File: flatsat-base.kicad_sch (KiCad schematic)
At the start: 11 parts, among them J1 xf2m-2415-1a-symbols, J10 Conn_01x24_Male, J11 Conn_02x05_Odd_Even, J12 Conn_02x05_Odd_Even, J13 Conn_01x10_Male, J3 XF2M-1015-1A-symbols, J4 XF2M-1015-1A-symbols, J5 XF2M-1015-1A-symbols, J6 XF2M-1015-1A-symbols, J7 XF2M-1015-1A-symbols, J8 XF2M-1015-1A-symbols

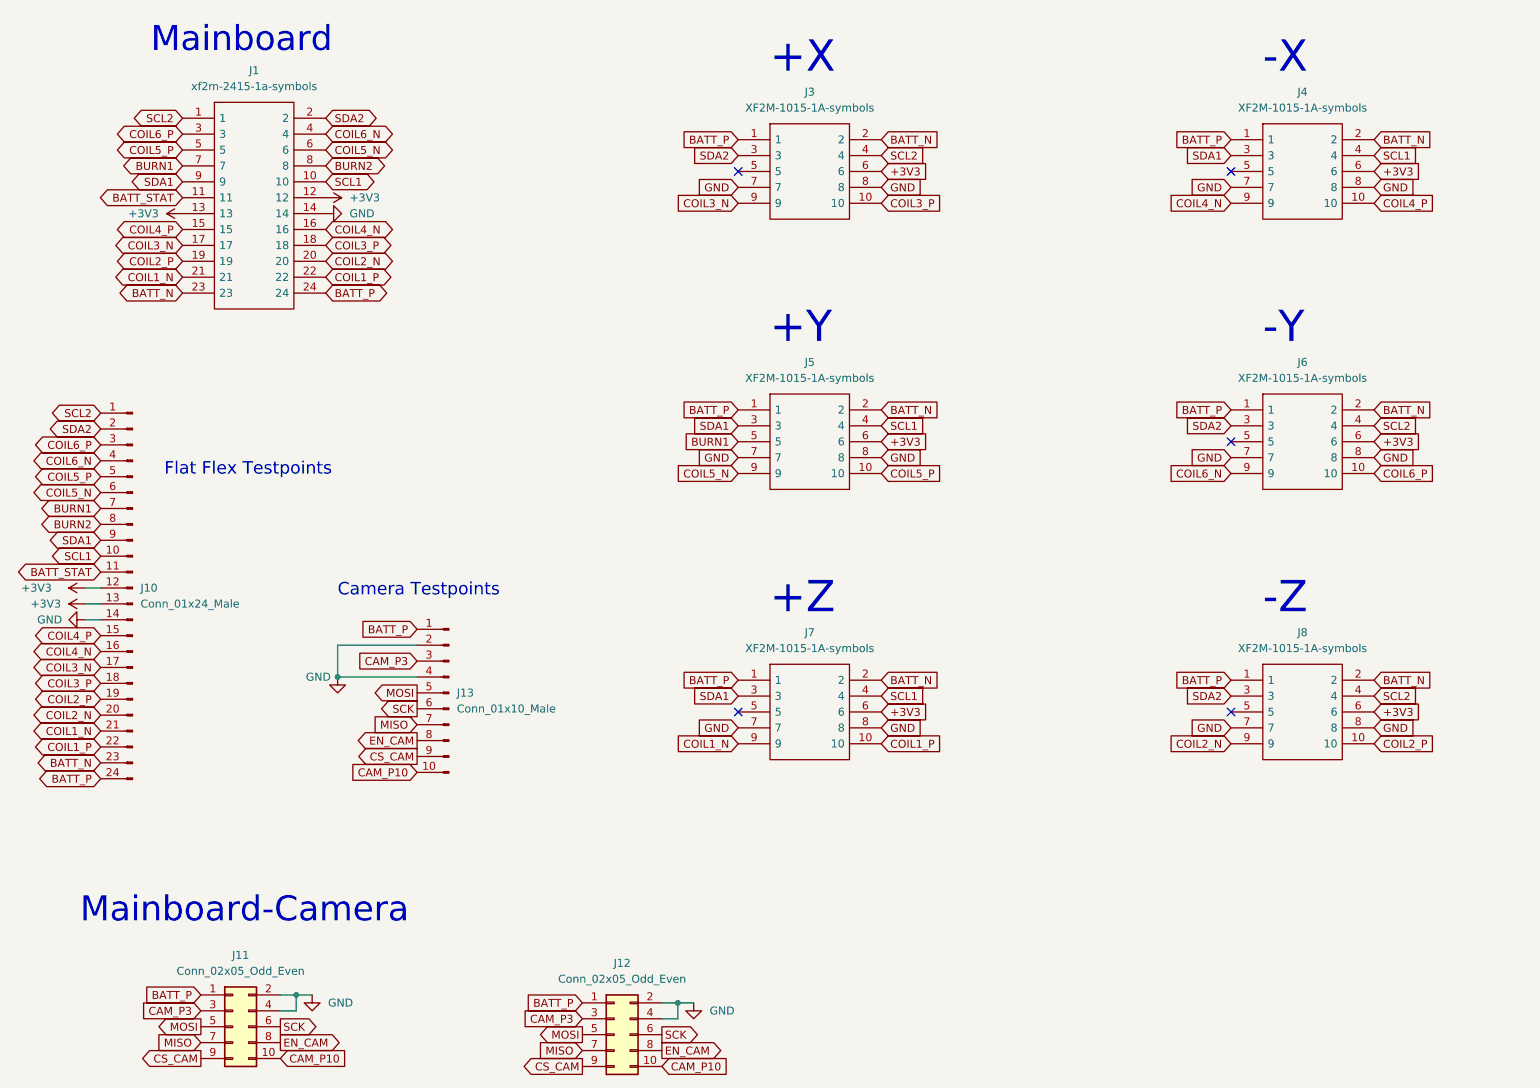
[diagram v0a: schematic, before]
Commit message: Partially routed
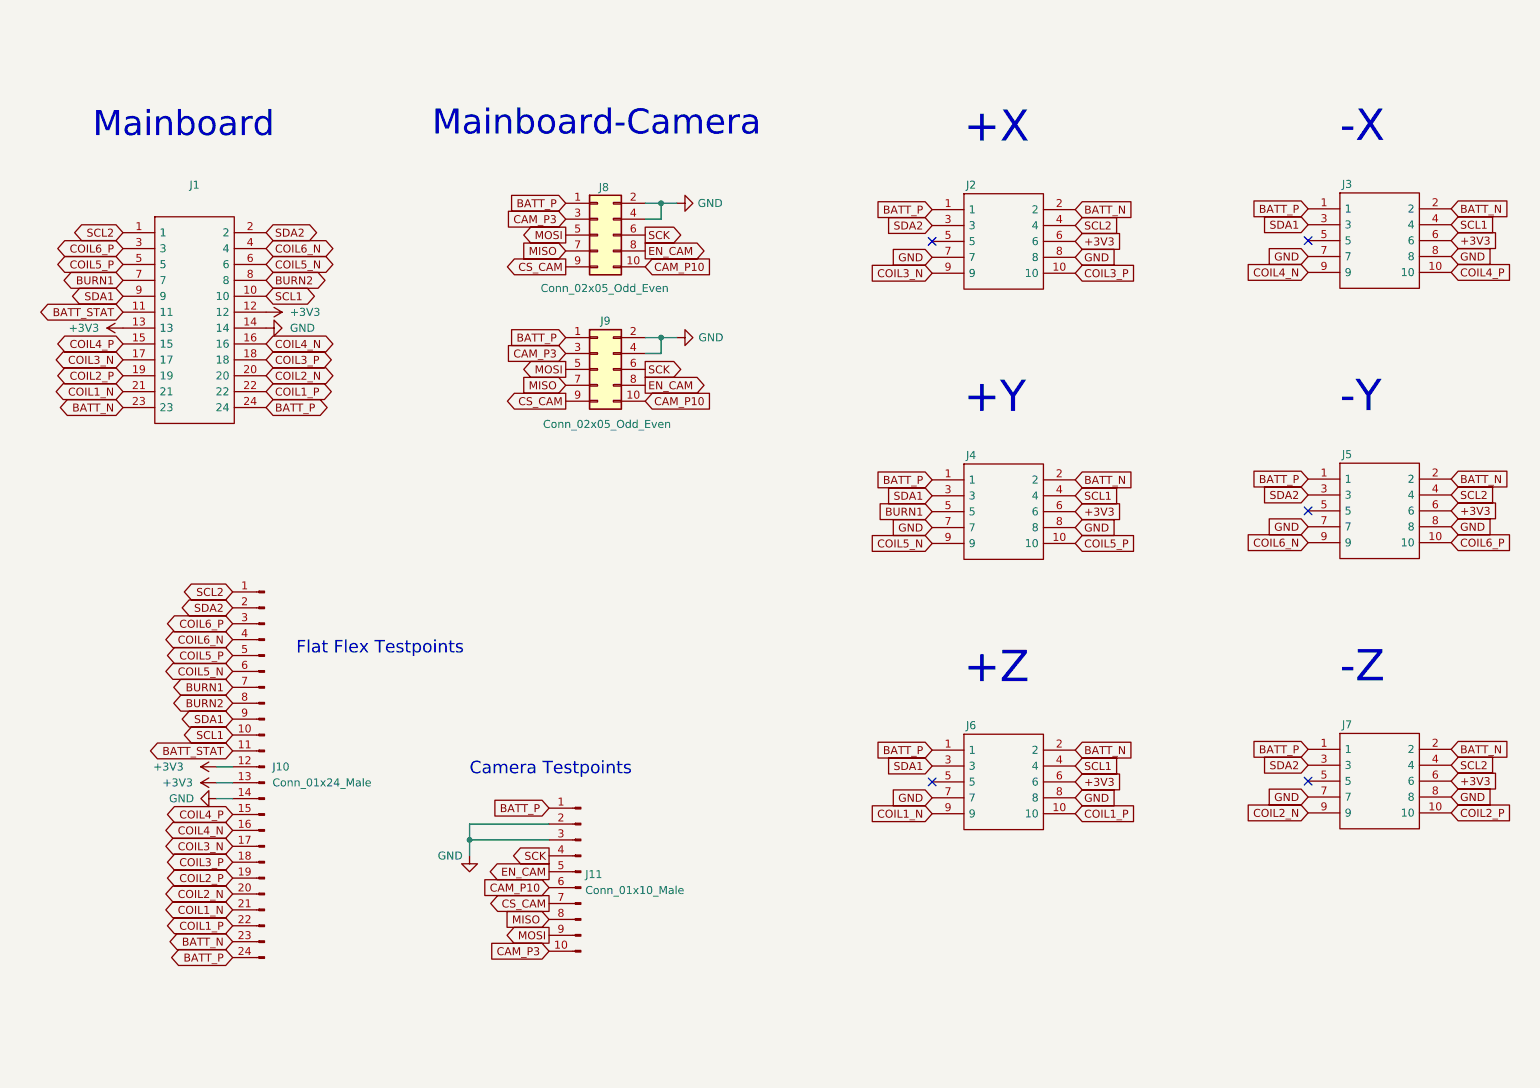
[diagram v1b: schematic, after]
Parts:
- J1: value xf2m-2415-1a-symbols -> (none); footprint PyCubed-Mini Main:XF2M-2415-1A -> (none); symbol PyCubed Mini avionics-motherboard:xf2m-2415-1a-symbols -> mainboard:FFC2B28-24-G
- J2: renamed from J3; value XF2M-1015-1A-symbols -> (none); footprint PyCubed-Mini Solar:XF2M-1015-1A -> solarpanels:GCT_FFC2B28-10-G; symbol PyCubed Mini avionics-motherboard:XF2M-1015-1A-symbols -> solarpanels:FFC2B28-10-G
- J3: renamed from J4; value XF2M-1015-1A-symbols -> (none); footprint PyCubed-Mini Solar:XF2M-1015-1A -> solarpanels:GCT_FFC2B28-10-G; symbol PyCubed Mini avionics-motherboard:XF2M-1015-1A-symbols -> solarpanels:FFC2B28-10-G
- J4: renamed from J5; value XF2M-1015-1A-symbols -> (none); footprint PyCubed-Mini Solar:XF2M-1015-1A -> solarpanels:GCT_FFC2B28-10-G; symbol PyCubed Mini avionics-motherboard:XF2M-1015-1A-symbols -> solarpanels:FFC2B28-10-G
- J5: renamed from J6; value XF2M-1015-1A-symbols -> (none); footprint PyCubed-Mini Solar:XF2M-1015-1A -> solarpanels:GCT_FFC2B28-10-G; symbol PyCubed Mini avionics-motherboard:XF2M-1015-1A-symbols -> solarpanels:FFC2B28-10-G
- J6: renamed from J7; value XF2M-1015-1A-symbols -> (none); footprint PyCubed-Mini Solar:XF2M-1015-1A -> solarpanels:GCT_FFC2B28-10-G; symbol PyCubed Mini avionics-motherboard:XF2M-1015-1A-symbols -> solarpanels:FFC2B28-10-G
- J7: renamed from J8; value XF2M-1015-1A-symbols -> (none); footprint PyCubed-Mini Solar:XF2M-1015-1A -> solarpanels:GCT_FFC2B28-10-G; symbol PyCubed Mini avionics-motherboard:XF2M-1015-1A-symbols -> solarpanels:FFC2B28-10-G
- J8: renamed from J11; footprint Connector_PinHeader_1.27mm:PinHeader_2x05_P1.27mm_Vertical -> (none)
- renumbered J13 to J11, J12 to J9
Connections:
- net CAM_P10: now also J11.6 (Pin_6); no longer J11.10 (Pin_10)
- net CAM_P3: now also J11.10 (Pin_10); no longer J11.3 (Pin_3)
- net CS_CAM: now also J11.7 (Pin_7); no longer J11.9 (Pin_9)
- net EN_CAM: now also J11.5 (Pin_5); no longer J11.8 (Pin_8)
- net GND: now also J11.3 (Pin_3); no longer J11.4 (Pin_4)
- net MISO: now also J11.8 (Pin_8); no longer J11.7 (Pin_7)
- net MOSI: now also J11.9 (Pin_9); no longer J11.5 (Pin_5)
- net SCK: now also J11.4 (Pin_4); no longer J11.6 (Pin_6)
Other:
- moved on the sheet: J1, J10, J11, J2, J3, J4, J5, J6, J7, J8, J9
